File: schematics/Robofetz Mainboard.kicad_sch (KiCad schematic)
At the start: 11 parts, among them J1 On/Off Switch, J2 Battery Connector, J3 Conn_01x04_Pin, J4 Motor 1, J5 Motor 2, J6 Weapon Controller, U2 DCDC, U3 ROB-14450

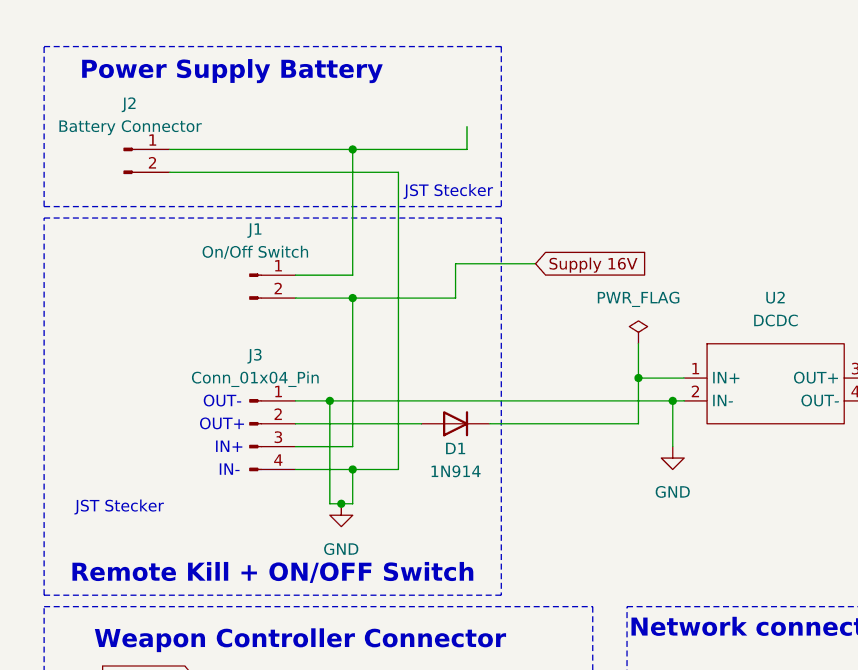
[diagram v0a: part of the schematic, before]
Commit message: updated schematics + layout
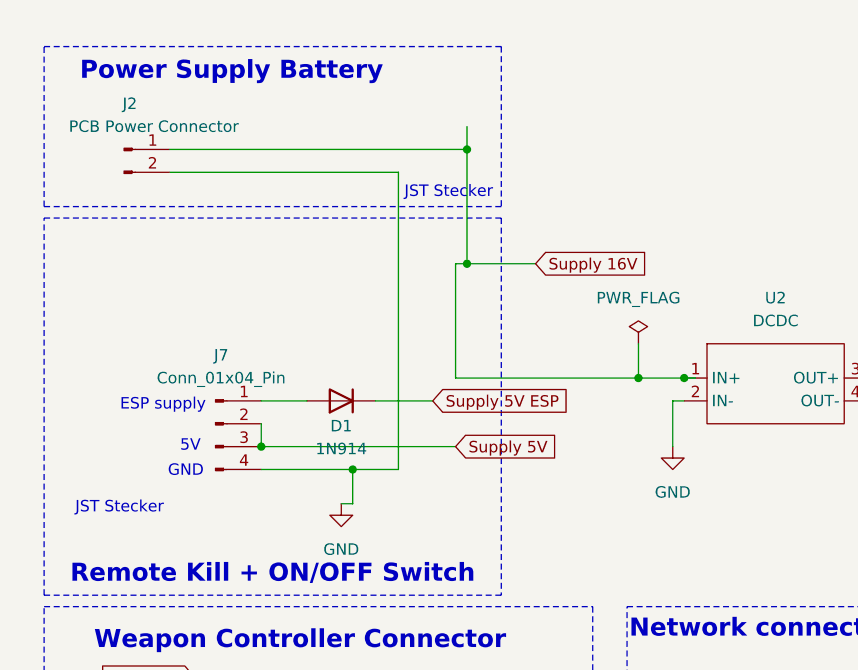
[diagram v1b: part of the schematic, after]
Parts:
- removed J1: On/Off Switch, Connector_JST:JST_EH_B2B-EH-A_1x02_P2.50mm_Vertical, symbol Connector:Conn_01x02_Pin
- removed J3: Conn_01x04_Pin, Connector_JST:JST_EH_B4B-EH-A_1x04_P2.50mm_Vertical, symbol Connector:Conn_01x04_Pin
- added J7: Conn_01x04_Pin, symbol Connector:Conn_01x04_Pin
- J2: value Battery Connector -> PCB Power Connector
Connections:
- net +5V: now also J7.2 (Pin_2), J7.3 (Pin_3)
- net GND: now also J7.4 (Pin_4)
- net Supply 16V: now also J2.1 (Pin_1), U2.1 (IN+)
- net Supply 5V ESP: now reaches D1.1 (K)
- net Supply 5V ESP: no longer U2.1 (IN+)
- net at D1.2 (A): now also J7.1 (Pin_1)
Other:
- note added: "5V"
- note added: "ESP supply"
- note added: "GND"
- note removed: "IN+"
- note removed: "IN-"
- note removed: "OUT+"
- note removed: "OUT-"
- moved on the sheet: D1
